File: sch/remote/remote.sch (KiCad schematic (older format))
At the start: 24 parts, among them J1 swd, J2 power_sw, J3 USB_A, Q1 DTD114E, U1 STM32F103C8Tx_usb, U2 XC6206-33, U3 TSOP17xx, Y1 8M

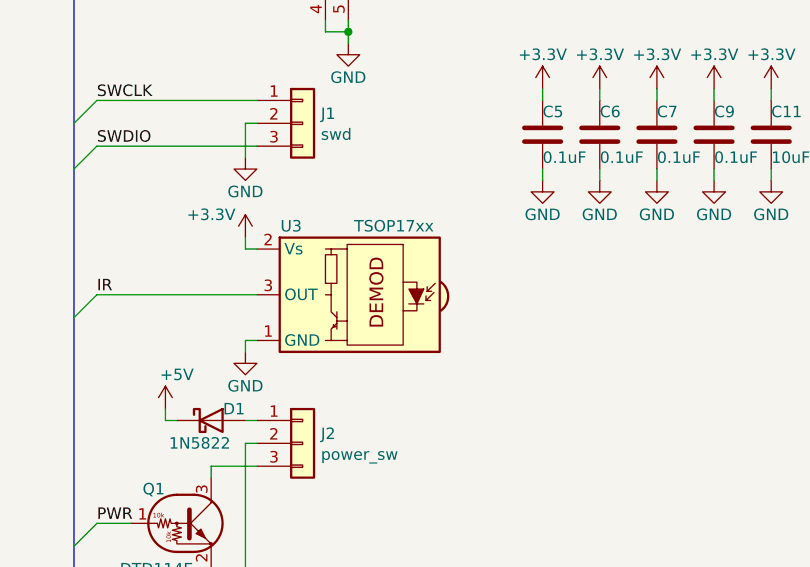
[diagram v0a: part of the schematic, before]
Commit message: убрался в файлах
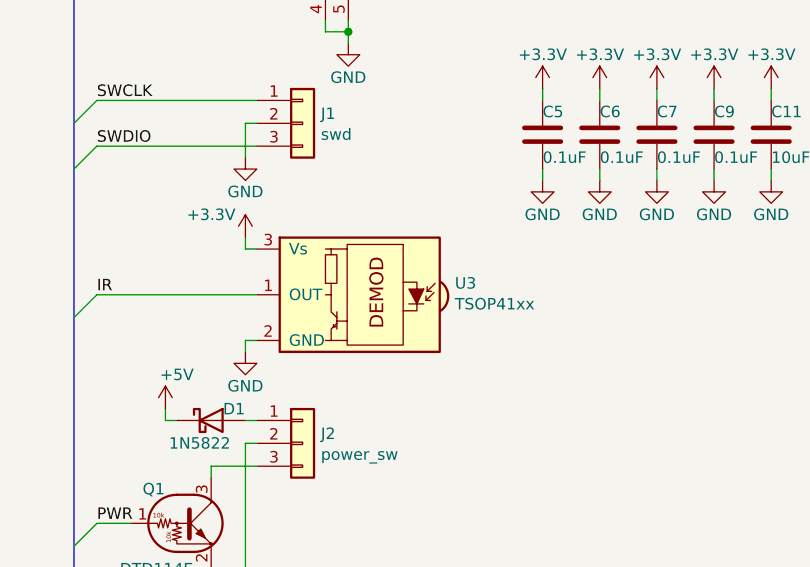
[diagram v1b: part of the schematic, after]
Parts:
- removed U3: TSOP17xx, OptoDevice:Vishay_CAST-3Pin, symbol Interface_Optical:TSOP17xx
- added U3: TSOP41xx, OptoDevice:Vishay_MOLD-3Pin, symbol Interface_Optical:TSOP41xx
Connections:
- net +3V3: now also U3.3 (Vs)
- net GND: now also U3.2 (GND)
- net IR: now also U3.1 (OUT)
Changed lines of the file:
@@
 	1    0    0    -1
-$EndComp
-$Comp
-L Interface_Optical:TSOP17xx U3
-U 1 1 61EC21C1
-P 7500 4450
-F 0 "U3" H 7750 4750 50  0000 C CNN
-F 1 "TSOP17xx" H 7300 4750 50  0000 C CNN
-F 2 "OptoDevice:Vishay_CAST-3Pin" H 7450 4075 50  0001 C CNN
-F 3 "http://www.micropik.com/PDF/tsop17xx.pdf" H 8150 4750 50  0001 C CNN
-	1    7500 4450
-	-1   0    0    -1
 $EndComp
 Wire Wire Line
@@
 NoConn ~ 4450 4400
 NoConn ~ 4450 4300
+Entry Wire Line
+	4100 4100 4200 4000
+Wire Wire Line
+	4200 4000 4450 4000
 Wire Bus Line
 	4150 5750 6450 5750
-Entry Wire Line
-	4100 4100 4200 4000
-Wire Wire Line
-	4200 4000 4450 4000
+$Comp
+L Interface_Optical:TSOP41xx U3
+U 1 1 625F74B2
+P 7500 4450
+F 0 "U3" H 7034 4500 50  0000 R CNN
+F 1 "TSOP41xx" H 7034 4409 50  0000 R CNN
+F 2 "OptoDevice:Vishay_MOLD-3Pin" H 7450 4075 50  0001 C CNN
+F 3 "http://www.vishay.com/docs/82460/tsop45.pdf" H 8150 4750 50  0001 C CNN
+	1    7500 4450
+	-1   0    0    -1
+$EndComp
 Wire Bus Line
 	4100 4050 4100 5700
